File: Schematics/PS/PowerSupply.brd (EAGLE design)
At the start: 157.5 x 127 mm, 79 parts, among them IC1 LM317MABDT, IC2 LM337, T1 IRFP240, T2 IRFP240

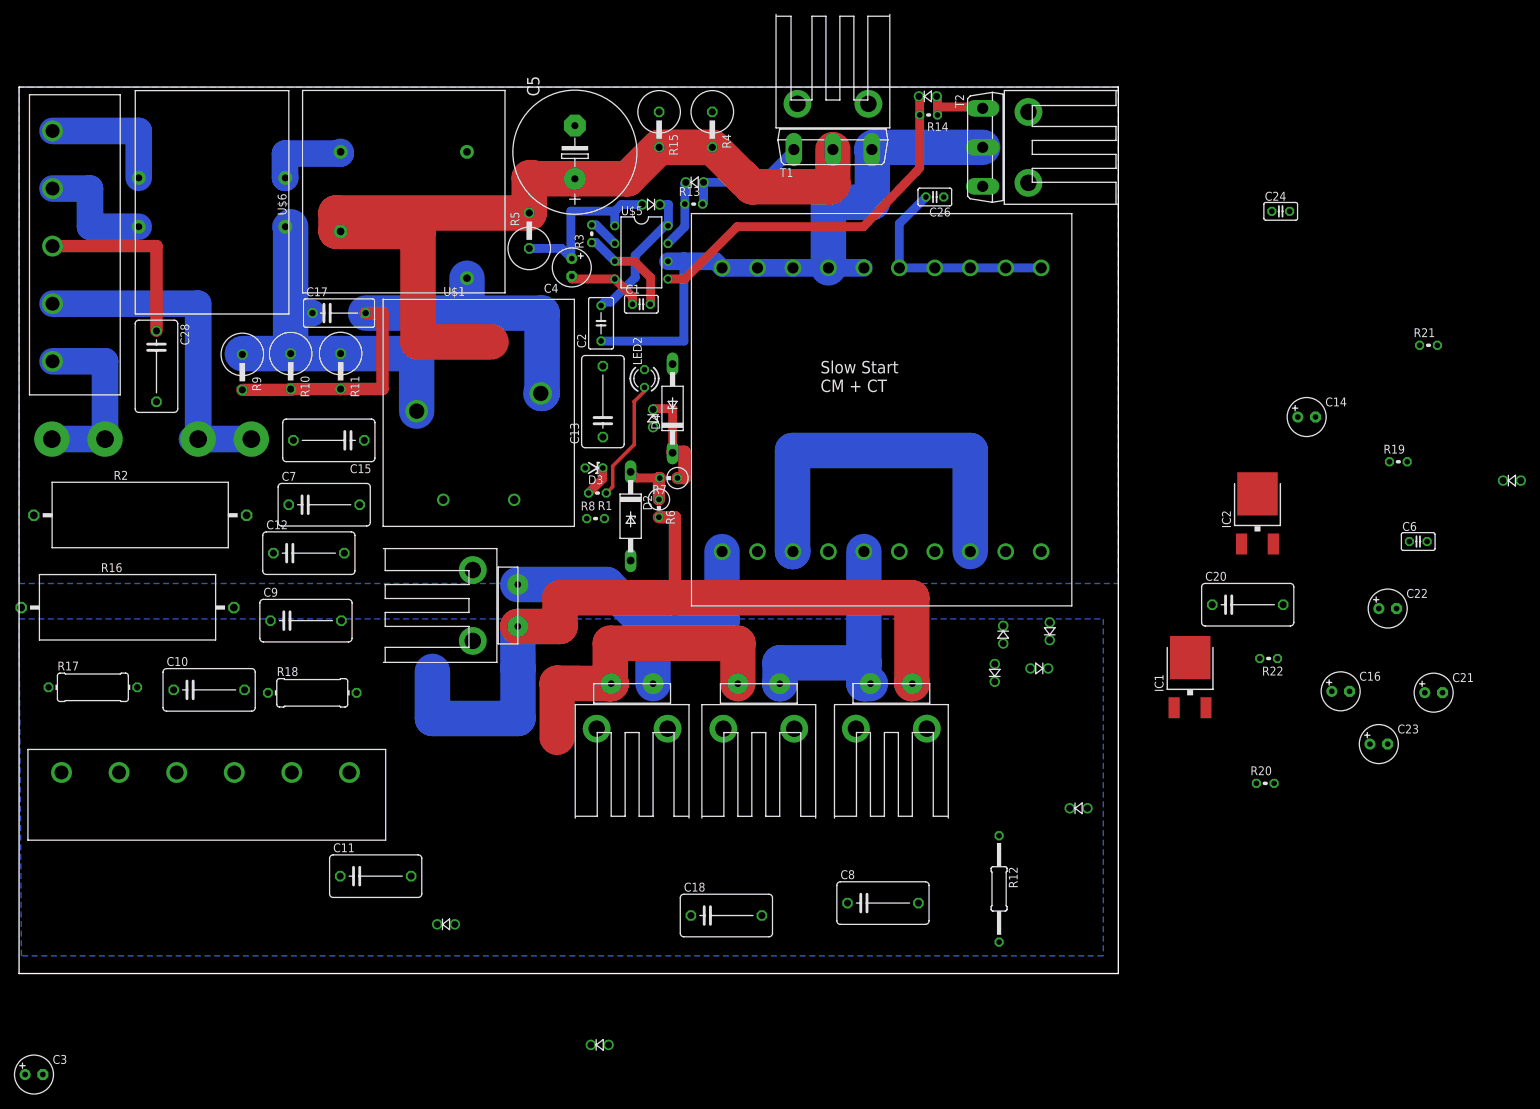
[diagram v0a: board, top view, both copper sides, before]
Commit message: updates to PS
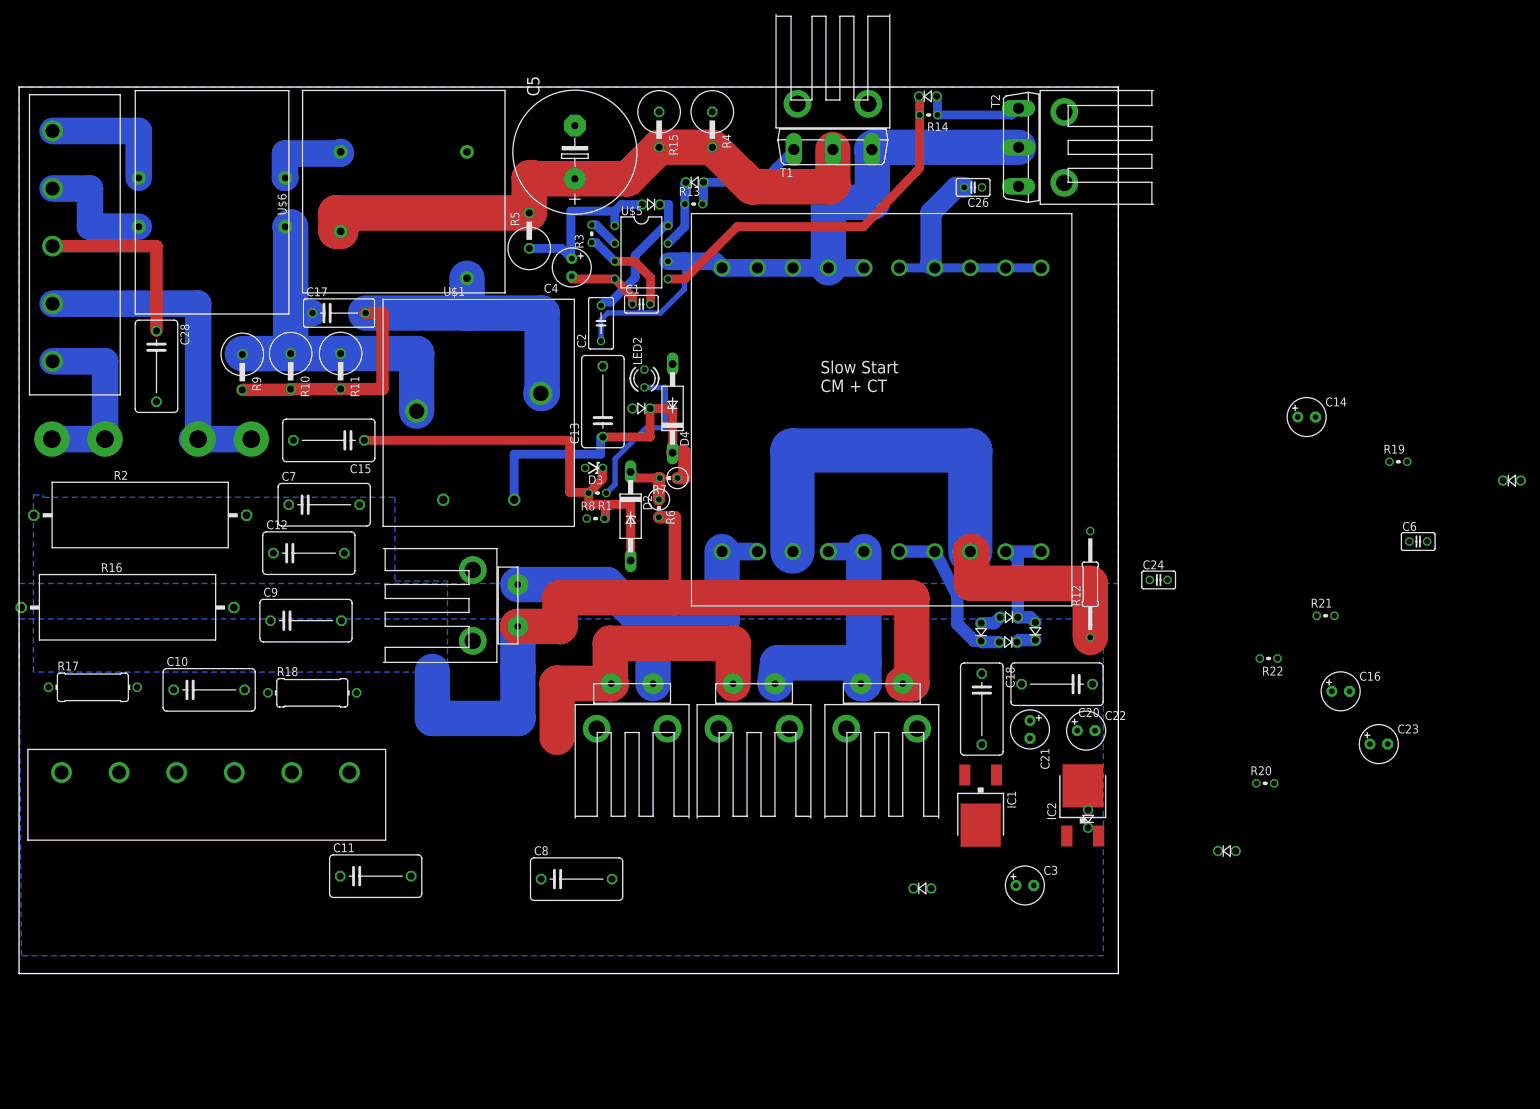
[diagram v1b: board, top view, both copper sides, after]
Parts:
- moved C3 144.5 mm to (144.1, 12.6)
- moved D11 94.0 mm to (170.2, 17.6)
- moved D18 68.4 mm to (126.6, 12.2)
- moved C21 58.1 mm to (144.8, 35.0), turned to 270 degrees
- moved C24 55.6 mm to (163.3, 56.4)
- moved IC2 48.8 mm to (152.4, 24.5)
- moved C18 47.1 mm to (137.9, 37.9), turned to 270 degrees
- moved C22 46.6 mm to (152.9, 34.8)
- moved R12 45.6 mm to (153.5, 55.8), turned to 90 degrees
- moved C8 44.0 mm to (79.9, 13.5)
- moved R21 41.5 mm to (187.2, 51.3)
- moved IC1 35.6 mm to (137.8, 23.6), turned to 180 degrees
- moved C20 29.6 mm to (148.7, 41.5), turned to 180 degrees
- moved D14 25.1 mm to (137.8, 46.1), turned to 90 degrees
- moved D17 24.8 mm to (153.2, 19.3)
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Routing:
- net MUTE: track 4.44 -> 62.0 mm
- net V+: track 128.5 -> 91.1 mm
- net N$10: track 15.6 -> 48.6 mm
- net SGND: track 54.5 -> 84.0 mm
- net VAC+15: track 0.00 -> 23.3 mm
- net VAC-15: track 0.00 -> 17.8 mm
- net N$1: track 17.4 -> 23.2 mm
- net N$21: track 9.27 -> 14.7 mm
- net VAC+40: track 50.0 -> 55.1 mm
- net VAC-40: track 34.9 -> 39.8 mm
- net V-15UN: track 0.00 -> 3.07 mm
- net V15UN: track 0.00 -> 2.74 mm
- net N$9: track 32.1 -> 34.8 mm
- net N$22: track 91.1 -> 93.7 mm
- net VCC: track 119.0 -> 120.2 mm
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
